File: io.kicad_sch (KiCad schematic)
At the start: 1 part, among them U1 STM32H723ZGTx

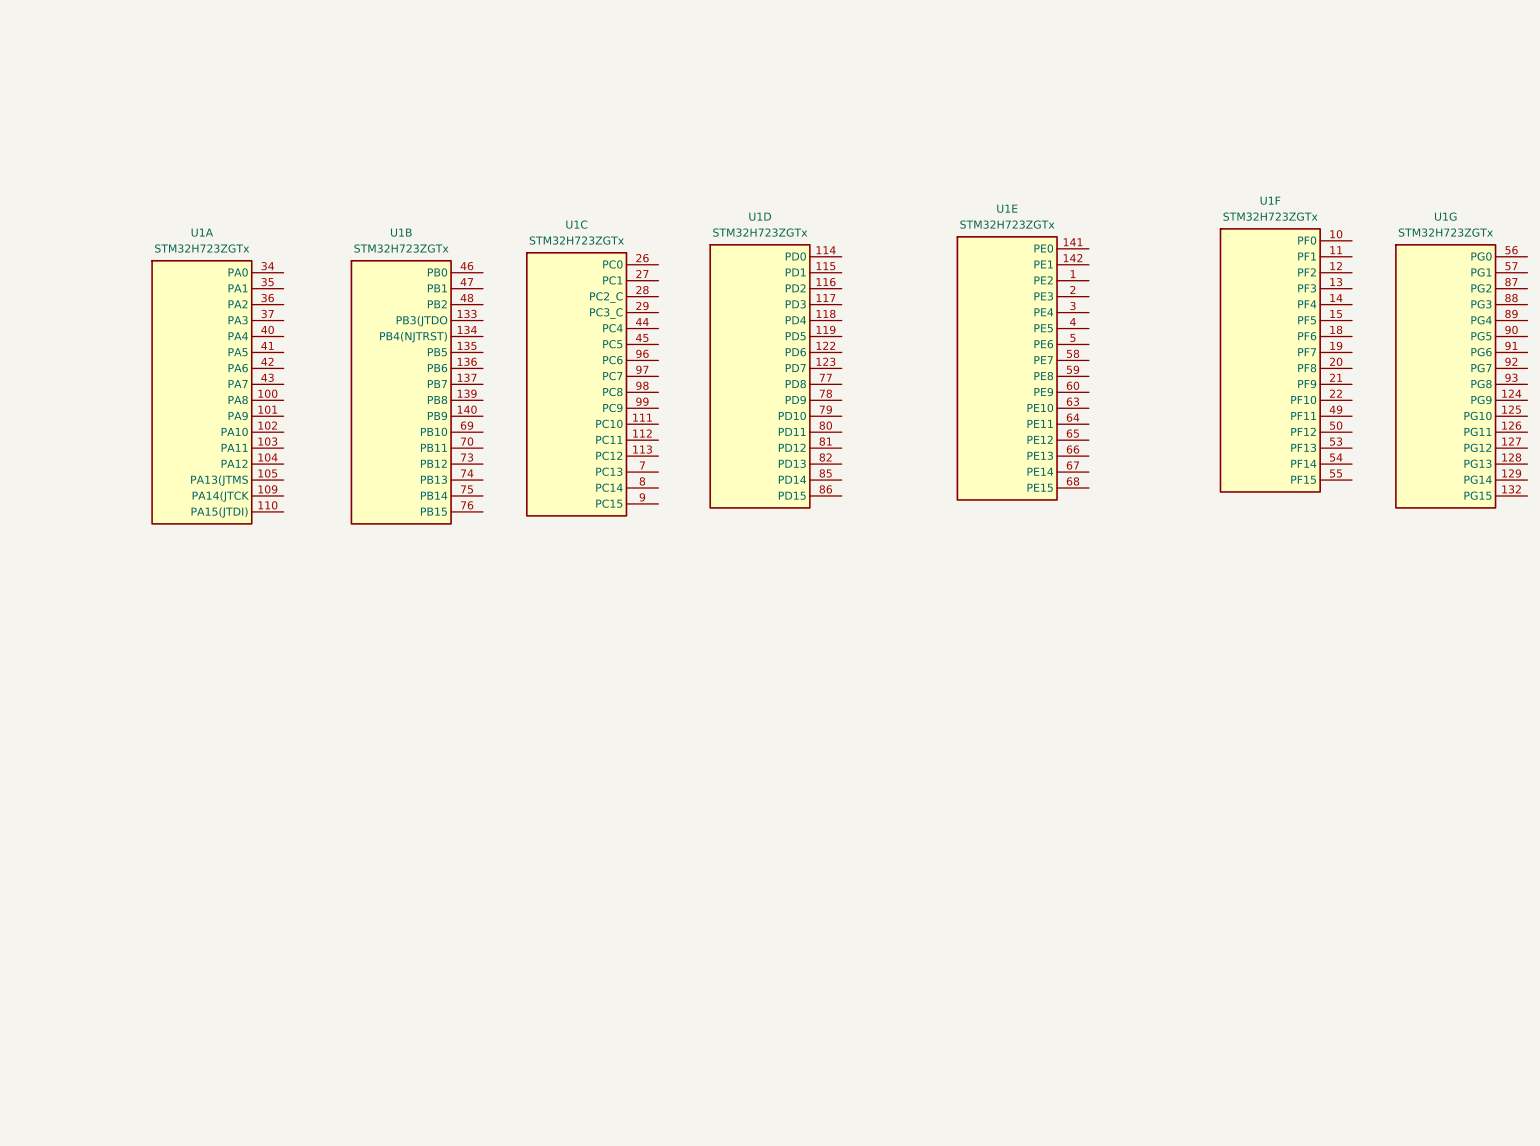
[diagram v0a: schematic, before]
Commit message: I dont know whats going on here
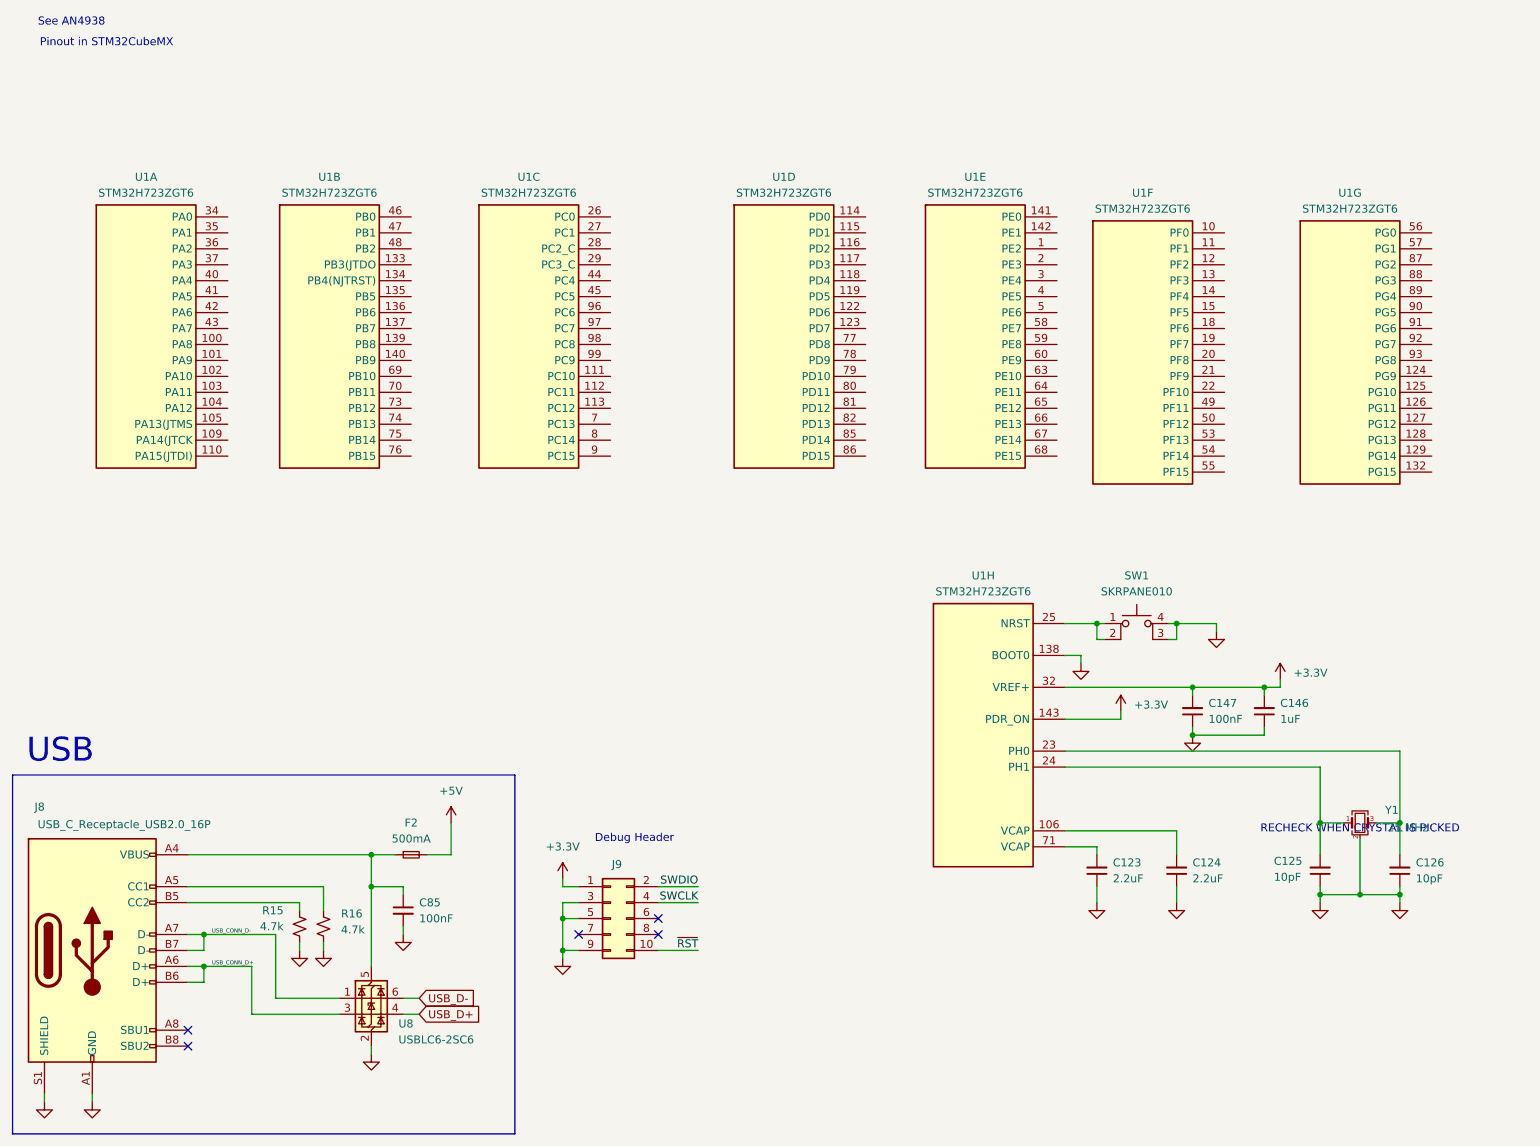
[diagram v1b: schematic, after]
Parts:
- added C123, C124: 2.2uF, symbol Device:C_Small
- added C125, C126: 10pF, symbol Device:C_Small
- added C146: 1uF, symbol Device:C_Small
- added C147: 100nF, symbol Device:C_Small
- added C85: 100nF, aprlprints:C_0603-noct, symbol Device:C_Small
- added F2: 500mA, Fuse:Fuse_0805_2012Metric, symbol Device:Fuse_Small
- added J8: USB_C_Receptacle_USB2.0_16P, Connector_USB:USB_C_Receptacle_HRO_TYPE-C-31-M-12, symbol Connector:USB_C_Receptacle_USB2.0_16P
- added J9: Conn_02x05_Odd_Even, Connector_PinHeader_2.54mm:PinHeader_2x05_P2.54mm_Vertical, symbol Connector_Generic:Conn_02x05_Odd_Even
- added R15, R16: 4.7k, aprlprints:R_0603-noct, symbol Device:R_Small_US
- added SW1: SKRPANE010, symbol Switch:SW_MEC_5E
- added unit 8 of U1
- added U8: USBLC6-2SC6, Package_TO_SOT_SMD:SOT-23-6, symbol Power_Protection:USBLC6-2SC6
- added Y1: 25 MHz, symbol Device:Crystal_GND24_Small
- U1: value STM32H723ZGTx -> STM32H723ZGT6
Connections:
- new net: C125.2, U1.24 (PH1), Y1.1
- new net: J8.B5 (CC2), R15.2
- new net: SW1.1, SW1.2, U1.25 (NRST)
- new net: C126.2, U1.23 (PH0), Y1.3
- new net: C85.1, F2.1, J8.A4 (VBUS), J8.A9 (VBUS), J8.B4 (VBUS), J8.B9 (VBUS), U8.5 (VBUS)
- new net: J8.A5 (CC1), R16.1
- new net: C124.2, U1.106 (VCAP)
- new net: C123.2, U1.71 (VCAP)
- new net +3.3V: C146.2, C147.2, J9.1 (Pin_1), U1.143 (PDR_ON), U1.32 (VREF+)
- new net +5V: F2.2
- new net GND: C123.1, C124.1, C125.1, C126.1, C146.1, C147.1, C85.2, J8.A1 (GND), J8.A12 (GND), J8.B1 (GND), J8.B12 (GND), J8.S1 (SHIELD), J9.3 (Pin_3), J9.5 (Pin_5), J9.9 (Pin_9), R15.1, R16.2, SW1.3 (K), SW1.4 (A), U1.138 (BOOT0), U8.2 (GND), Y1.2 (G), Y1.4 (G)
- new net SWCLK: J9.4 (Pin_4)
- new net SWDIO: J9.2 (Pin_2)
- new net USB_CONN_D+: J8.A6 (D+), J8.B6 (D+), U8.3 (I/O2)
- new net USB_CONN_D-: J8.A7 (D-), J8.B7 (D-), U8.1 (I/O1)
- new net USB_D+: U8.4 (I/O2)
- new net USB_D-: U8.6 (I/O1)
- new net ~{RST}: J9.10 (Pin_10)
- no-connect marks 0 -> 5
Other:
- note added: "Debug Header"
- note added: "Pinout in STM32CubeMX"
- note added: "RECHECK WHEN CRYSTAL IS PICKED"
- note added: "See AN4938"
- note added: "USB"
